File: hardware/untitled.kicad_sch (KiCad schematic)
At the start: 4 parts

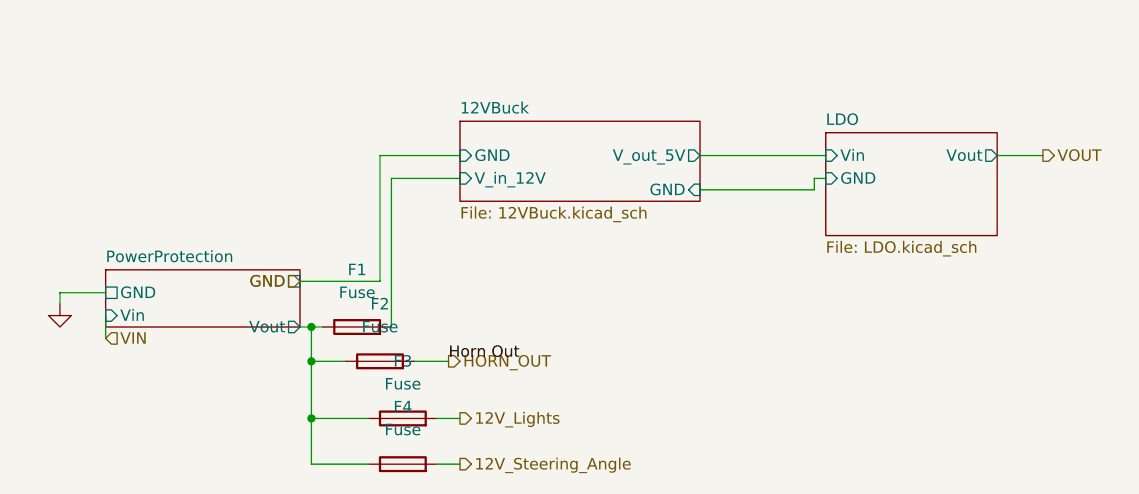
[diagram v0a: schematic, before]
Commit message: techuri
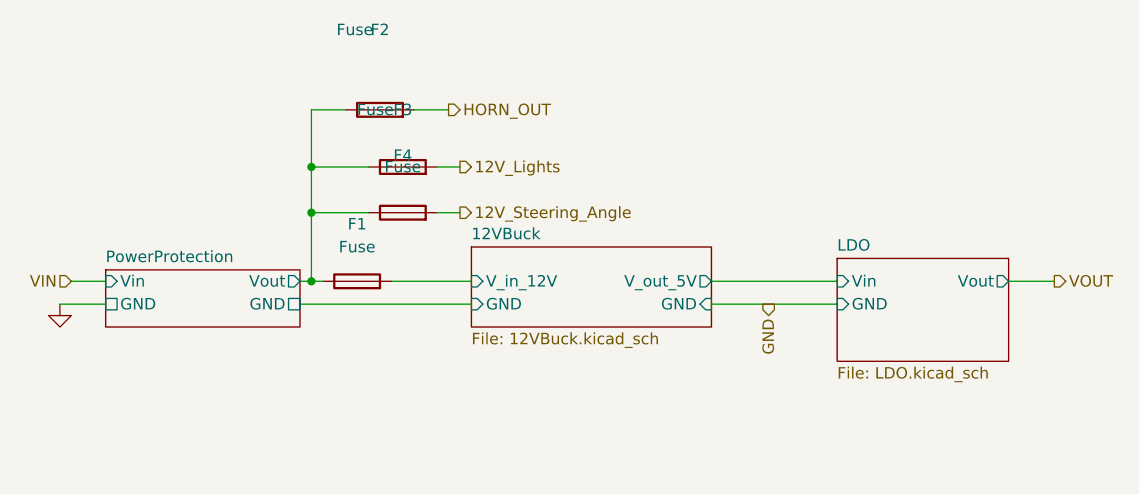
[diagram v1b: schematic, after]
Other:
- moved on the sheet: F1, F2, F3, F4
